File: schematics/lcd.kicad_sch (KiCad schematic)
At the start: 4 parts, among them U16 ATF22V10C-7, U24 74HC373

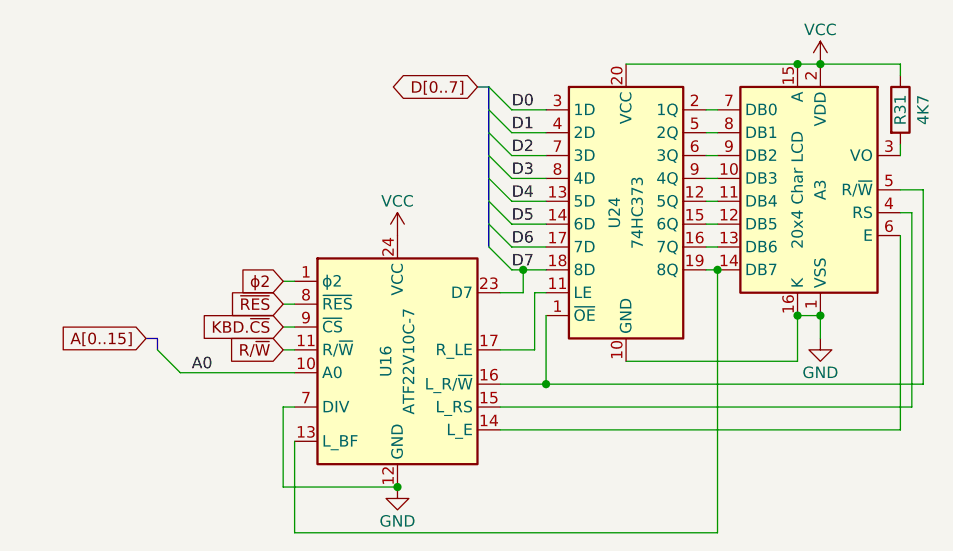
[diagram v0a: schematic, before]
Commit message: added phi0 for write latch timing
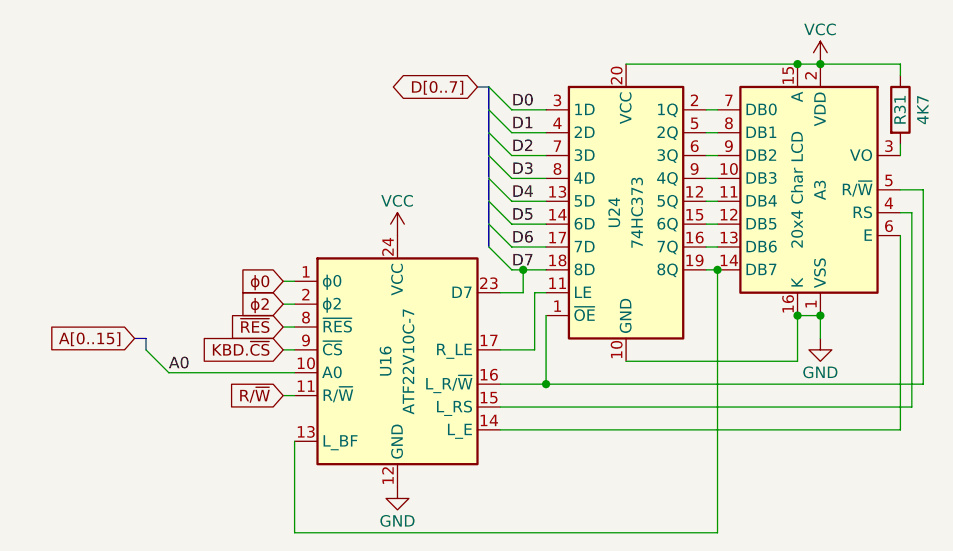
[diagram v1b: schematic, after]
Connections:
- net GND: no longer U16.7 (DIV)
- net ϕ2: now also U16.2 (ϕ2); no longer U16.1 (ϕ2)
- new net ϕ0: U16.1 (ϕ0)
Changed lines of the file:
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@@
-	)
-	(junction
-		(at 116.84 121.92)
-		(diameter 0)
-		(color 0 0 0 0)
 	)
 	(junction
@@
 	)
 	(bus_entry
-		(at 90.17 106.68)
+		(at 88.9 106.68)
 		(size 2.54 2.54)
 		(stroke
@@
 	(bus
 		(pts
-			(xy 90.17 105.41) (xy 90.17 106.68)
+			(xy 88.9 105.41) (xy 88.9 106.68)
 		)
 		(stroke
@@
 	(wire
 		(pts
-			(xy 92.71 109.22) (xy 105.41 109.22)
+			(xy 91.44 109.22) (xy 105.41 109.22)
 		)
 		(stroke
@@
 	(wire
 		(pts
-			(xy 104.14 121.92) (xy 116.84 121.92)
-		)
-		(stroke
-			(width 0)
-			(type default)
-		)
-	)
-	(wire
-		(pts
 			(xy 172.72 74.93) (xy 163.83 74.93)
 		)
@@
 		)
 	)
+	(wire
+		(pts
+			(xy 104.14 101.6) (xy 105.41 101.6)
+		)
+		(stroke
+			(width 0)
+			(type default)
+		)
+	)
 	(bus
 		(pts
@@
 		)
 	)
-	(wire
-		(pts
-			(xy 105.41 113.03) (xy 104.14 113.03)
-		)
-		(stroke
-			(width 0)
-			(type default)
-		)
-	)
 	(bus
 		(pts
@@
 	(wire
 		(pts
+			(xy 104.14 111.76) (xy 105.41 111.76)
+		)
+		(stroke
+			(width 0)
+			(type default)
+		)
+	)
+	(wire
+		(pts
 			(xy 129.54 97.79) (xy 130.81 97.79)
 		)
@@
 	(wire
 		(pts
+			(xy 104.14 104.14) (xy 105.41 104.14)
+		)
+		(stroke
+			(width 0)
+			(type default)
+		)
+	)
+	(wire
+		(pts
 			(xy 161.29 107.95) (xy 161.29 102.87)
 		)
@@
 	(bus
 		(pts
-			(xy 88.9 105.41) (xy 90.17 105.41)
+			(xy 87.63 105.41) (xy 88.9 105.41)
 		)
 		(stroke
@@
 	(wire
 		(pts
+			(xy 104.14 106.68) (xy 105.41 106.68)
+		)
+		(stroke
+			(width 0)
+			(type default)
+		)
+	)
+	(wire
+		(pts
 			(xy 172.72 93.98) (xy 172.72 115.57)
 		)
@@
 	(wire
 		(pts
-			(xy 104.14 106.68) (xy 105.41 106.68)
-		)
-		(stroke
-			(width 0)
-			(type default)
-		)
-	)
-	(wire
-		(pts
 			(xy 161.29 102.87) (xy 163.83 102.87)
 		)
@@
 	(wire
 		(pts
-			(xy 104.14 101.6) (xy 105.41 101.6)
-		)
-		(stroke
-			(width 0)
-			(type default)
-		)
-	)
-	(wire
-		(pts
 			(xy 129.54 90.17) (xy 133.35 90.17)
 		)
@@
 	(wire
 		(pts
-			(xy 104.14 104.14) (xy 105.41 104.14)
-		)
-		(stroke
-			(width 0)
-			(type default)
-		)
-	)
-	(wire
-		(pts
 			(xy 129.54 87.63) (xy 133.35 87.63)
 		)
@@
 		(pts
 			(xy 129.54 92.71) (xy 133.35 92.71)
-		)
-		(stroke
-			(width 0)
-			(type default)
-		)
-	)
-	(wire
-		(pts
-			(xy 104.14 113.03) (xy 104.14 121.92)
 		)
 		(stroke
@@
 	)
 	(label "A0"
-		(at 93.98 109.22 0)
+		(at 91.44 109.22 0)
 		(effects
 			(font
@@
 	(global_label "R{slash}~{W}"
 		(shape input)
-		(at 104.14 106.68 180)
+		(at 104.14 111.76 180)
 		(fields_autoplaced yes)
 		(effects
@@
 		)
 		(property "Intersheetrefs" "${INTERSHEET_REFS}"
-			(at 97.1029 106.68 0)
+			(at 97.1029 111.76 0)
 			(hide yes)
 			(show_name no)
@@
 	(global_label "A[0..15]"
 		(shape input)
-		(at 88.9 105.41 180)
+		(at 87.63 105.41 180)
 		(fields_autoplaced yes)
 		(effects
@@
 		)
 		(property "Intersheetrefs" "${INTERSHEET_REFS}"
-			(at 78.2947 105.41 0)
+			(at 77.0247 105.41 0)
 			(hide yes)
 			(show_name no)
@@
 		)
 	)
-	(global_label "ϕ2"
+	(global_label "ϕ0"
 		(shape input)
 		(at 104.14 99.06 180)
@@
 		)
 	)
-	(global_label "KBD.~{CS}"
+	(global_label "ϕ2"
 		(shape input)
-		(at 104.14 104.14 180)
+		(at 104.14 101.6 180)
 		(fields_autoplaced yes)
 		(effects
@@
 		)
 		(property "Intersheetrefs" "${INTERSHEET_REFS}"
-			(at 94.2605 104.14 0)
+			(at 98.6148 101.6 0)
 			(hide yes)
 			(show_name no)
@@
 		)
 	)
+	(global_label "KBD.~{CS}"
+		(shape input)
+		(at 104.14 106.68 180)
+		(fields_autoplaced yes)
+		(effects
+			(font
+				(size 1.27 1.27)
+			)
+			(justify right)
+		)
+		(property "Intersheetrefs" "${INTERSHEET_REFS}"
+			(at 94.2605 106.68 0)
+			(hide yes)
+			(show_name no)
+			(do_not_autoplace no)
+			(effects
+				(font
+					(size 1.27 1.27)
+				)
+				(justify right)
+			)
+		)
+	)
 	(global_label "~{RES}"
 		(shape input)
-		(at 104.14 101.6 180)
+		(at 104.14 104.14 180)
 		(fields_autoplaced yes)
 		(effects
@@
 		)
 		(property "Intersheetrefs" "${INTERSHEET_REFS}"
-			(at 97.5263 101.6 0)
+			(at 97.5263 104.14 0)
 			(hide yes)
 			(show_name no)
